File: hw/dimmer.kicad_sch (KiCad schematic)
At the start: 40 parts, among them J4 Screw_Terminal_01x02, Q10 MMBT3904, Q11 MMBT3906, Q13 IPN80R900P7, Q14 IPN80R900P7, Q9 MMBT3904, U2 PC817XI, U3 H11L1SR2M, U4 PC817XI

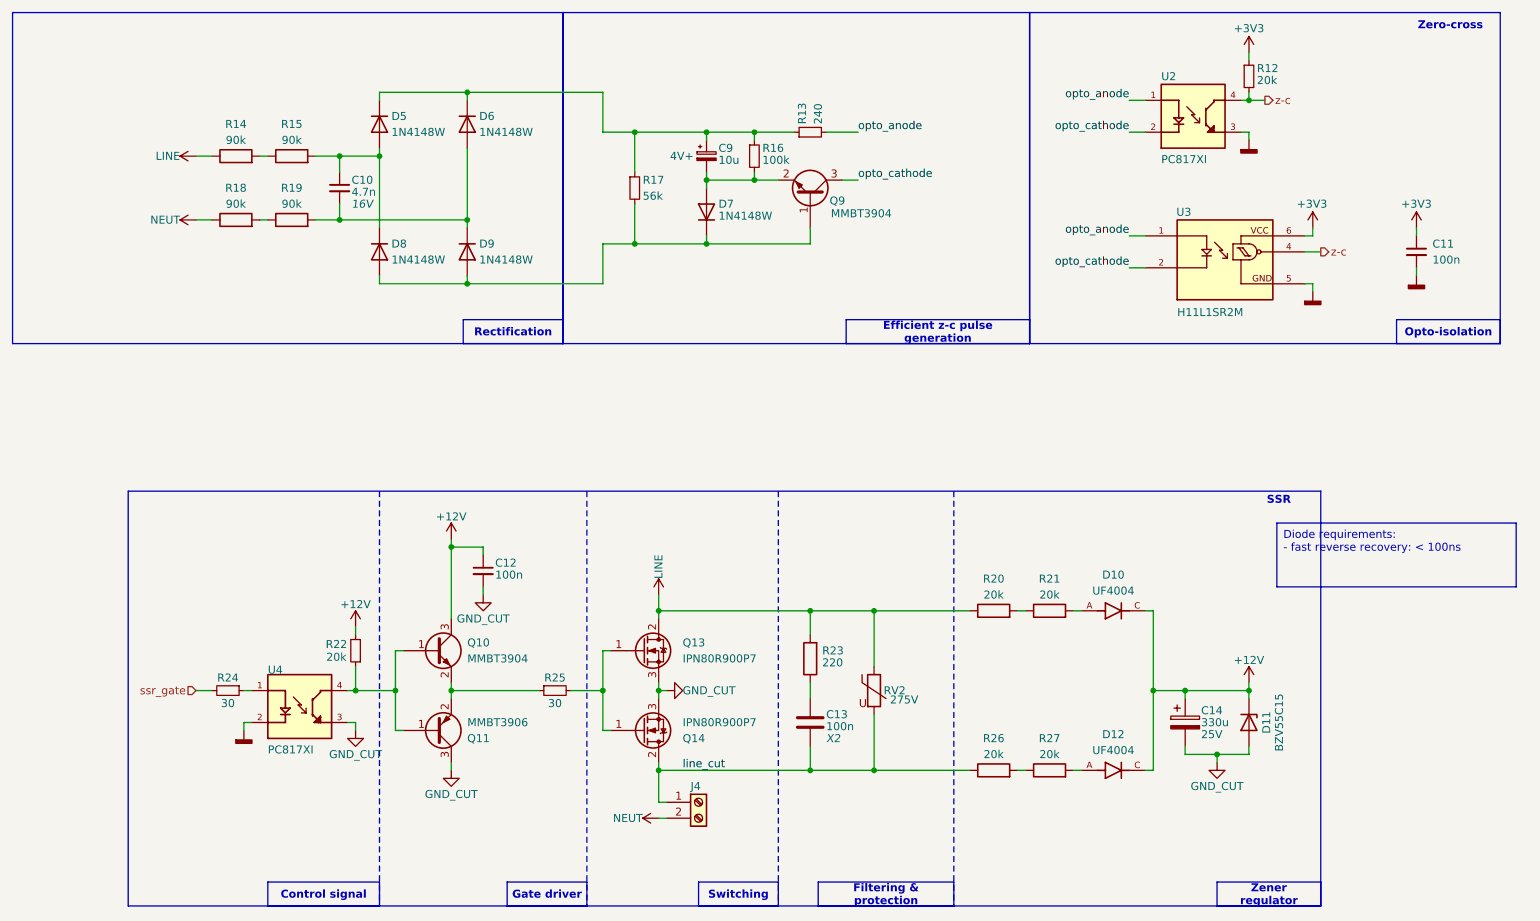
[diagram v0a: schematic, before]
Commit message: Update design
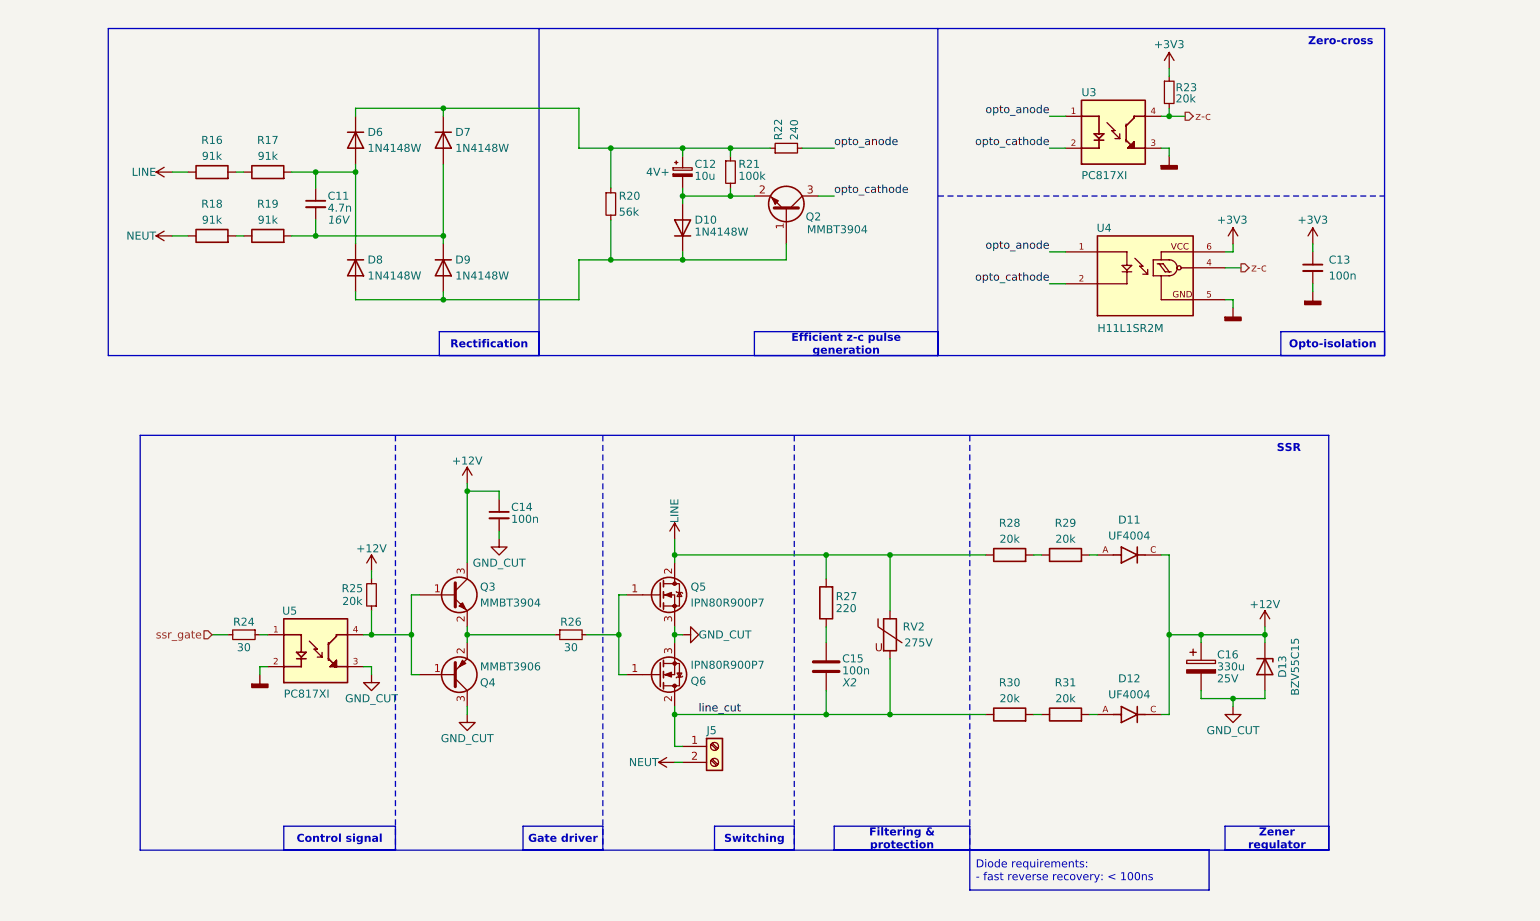
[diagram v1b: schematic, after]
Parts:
- R16: renamed from R14; value 90k -> 91k
- R17: renamed from R15; value 90k -> 91k
- R18, R19: value 90k -> 91k
- renumbered C10 to C11, C9 to C12, C11 to C13, C12 to C14, C13 to C15, C14 to C16, D7 to D10, D10 to D11, D11 to D13, D5 to D6, D6 to D7, J4 to J5, Q9 to Q2, Q10 to Q3, Q11 to Q4, Q13 to Q5, Q14 to Q6, R17 to R20, R16 to R21, R13 to R22, R12 to R23, R22 to R25, R25 to R26, R23 to R27, R20 to R28, R21 to R29, R26 to R30, R27 to R31, U2 to U3, U3 to U4, U4 to U5
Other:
- title: LEDDs -> Dimmer
- moved on the sheet: C11, C12, C13, C14, C15, C16, D10, D11, D12, D13, D6, D7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
